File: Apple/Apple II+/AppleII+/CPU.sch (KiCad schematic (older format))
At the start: 19 parts, among them U3 MOS6502

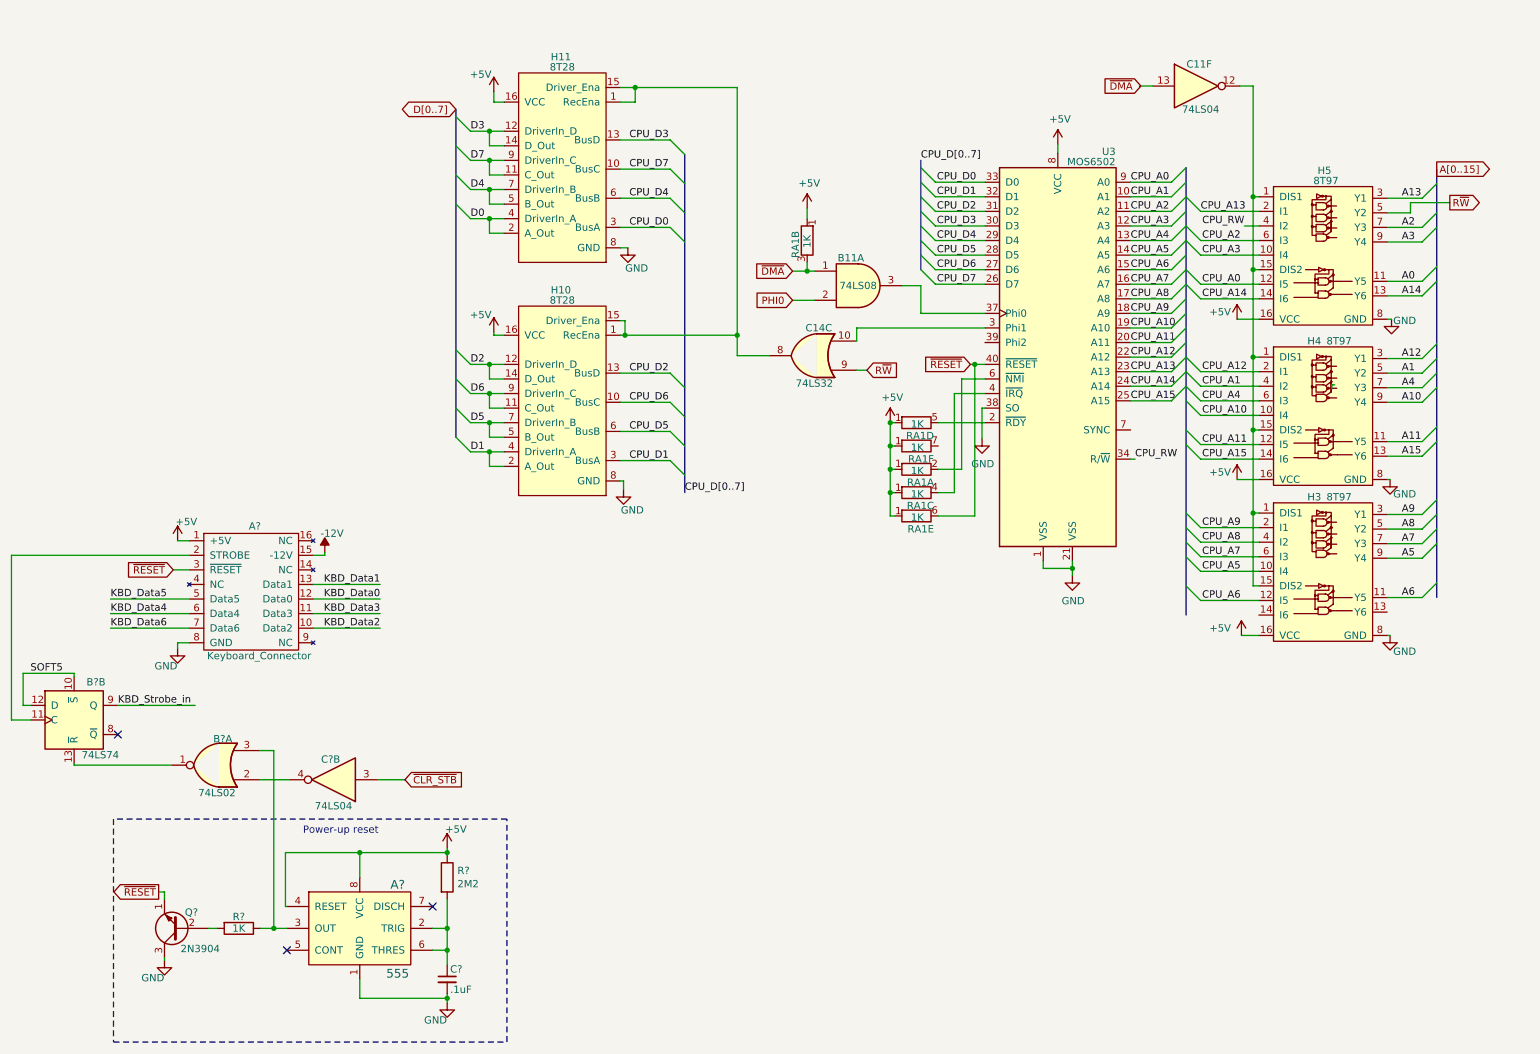
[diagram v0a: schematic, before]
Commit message: updated additional sheets, and Readme.md
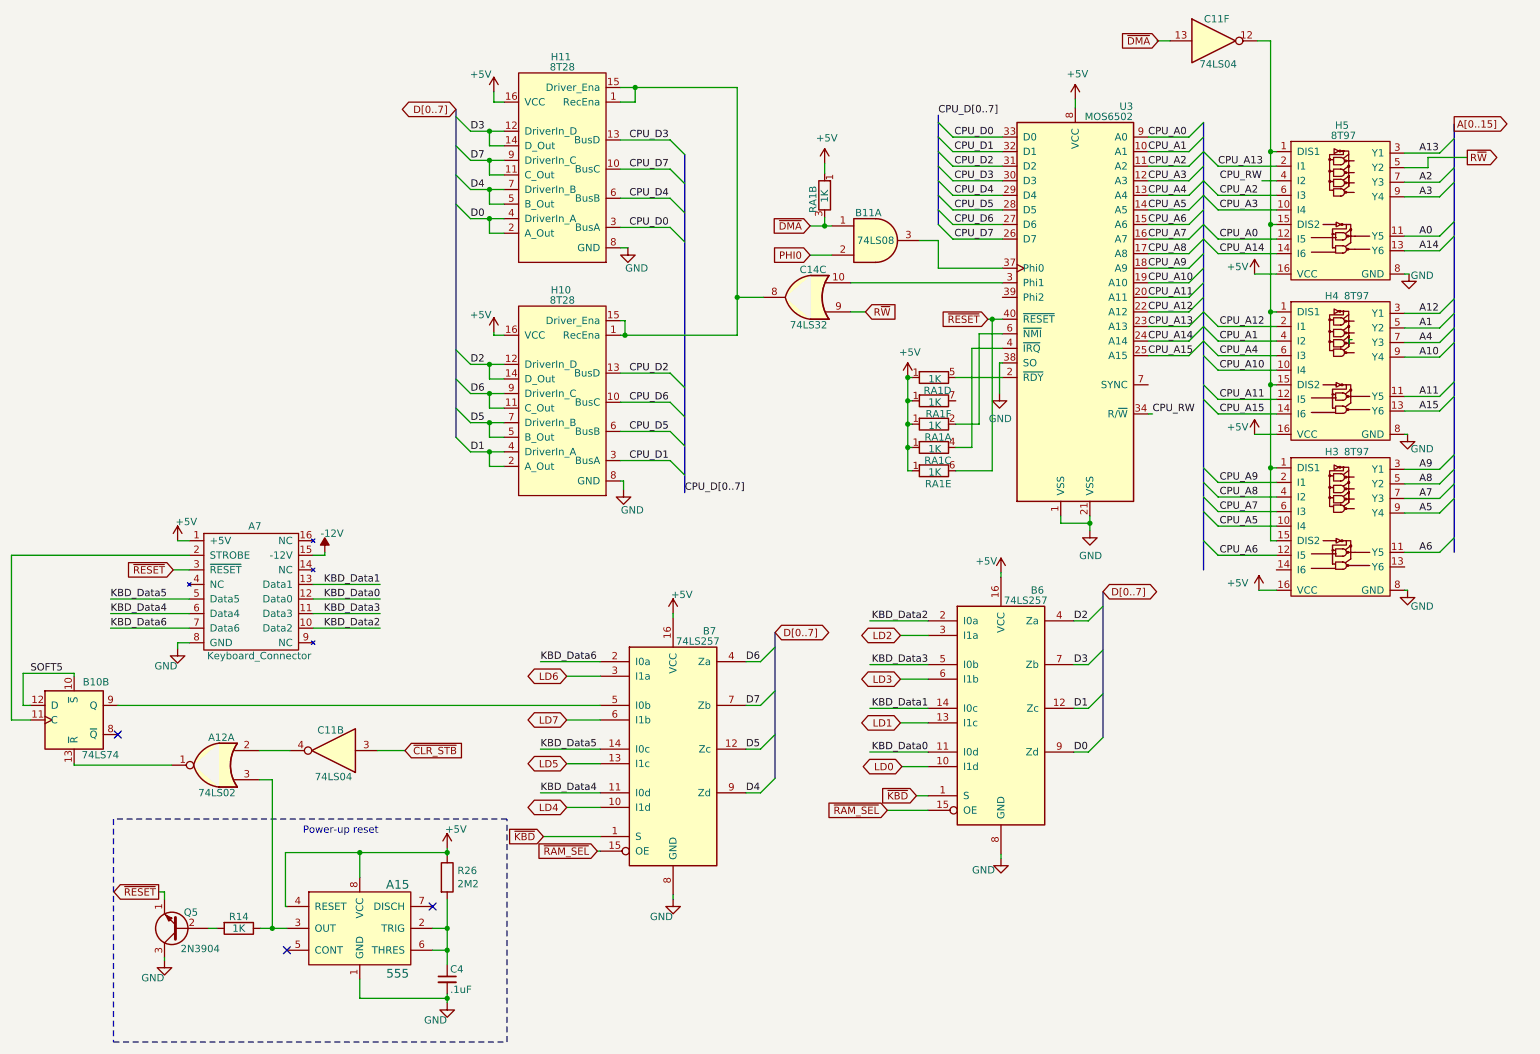
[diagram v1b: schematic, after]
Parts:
- added B6, B7: 74LS257, symbol 74xx:74LS257
- gave numbers to parts that had none: 9
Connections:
- net labels added: LD0, LD1, LD2, LD3, LD4, LD5, LD6, LD7, ~KBD, ~RAM_SEL
- net labels removed: KBD_Strobe_in
- wire segments 228 -> 258
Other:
- moved on the sheet: B11A, C11B, C11F, C14C, H3, H4, H5, RA1A, RA1B, RA1C, RA1D, RA1E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
